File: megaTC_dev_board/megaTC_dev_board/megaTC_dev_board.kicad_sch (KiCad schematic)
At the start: 20 parts, among them J1 Screw_Terminal_01x02, J10 Screw_Terminal_01x02, J11 Conn_01x06_Pin, J12 Screw_Terminal_01x02, J2 Screw_Terminal_01x02, J3 Screw_Terminal_01x02, J4 Screw_Terminal_01x02, J5 Screw_Terminal_01x02, J6 Screw_Terminal_01x02, J7 Screw_Terminal_01x02, J8 Screw_Terminal_01x02, J9 Screw_Terminal_01x02, U1 LTC2984CLX-PBF

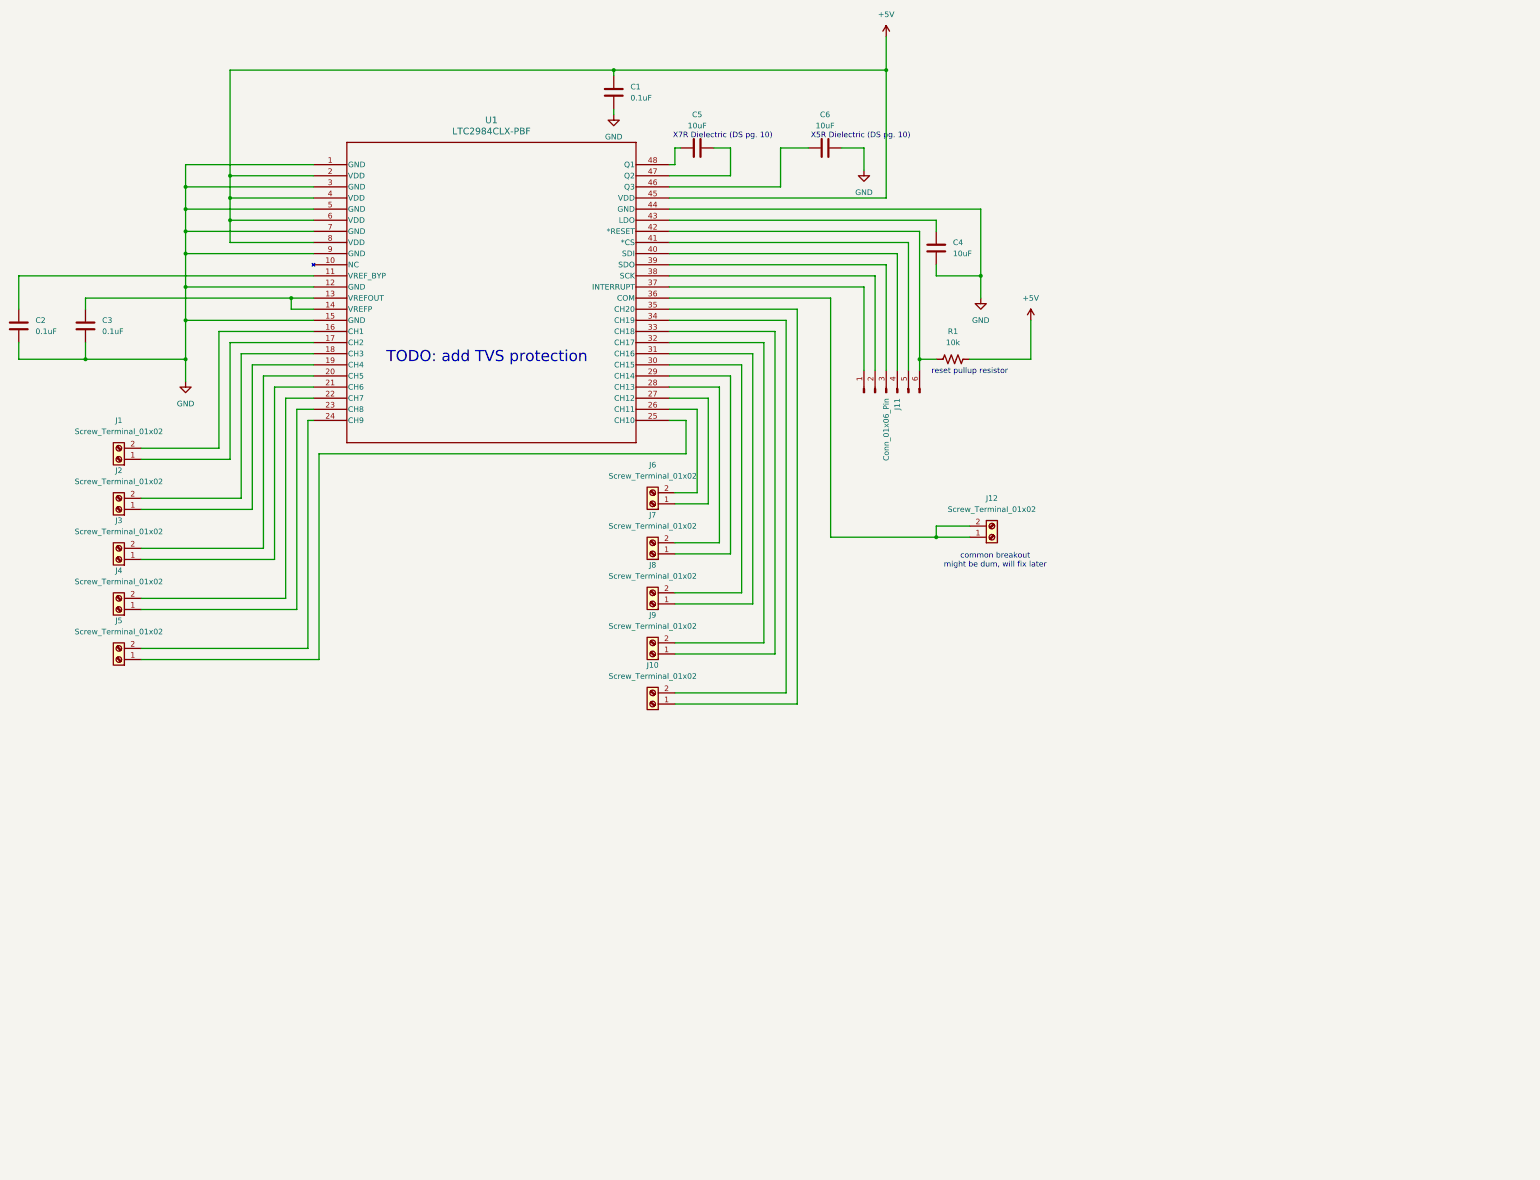
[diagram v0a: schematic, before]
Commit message: added TVS diodes, ready for routing
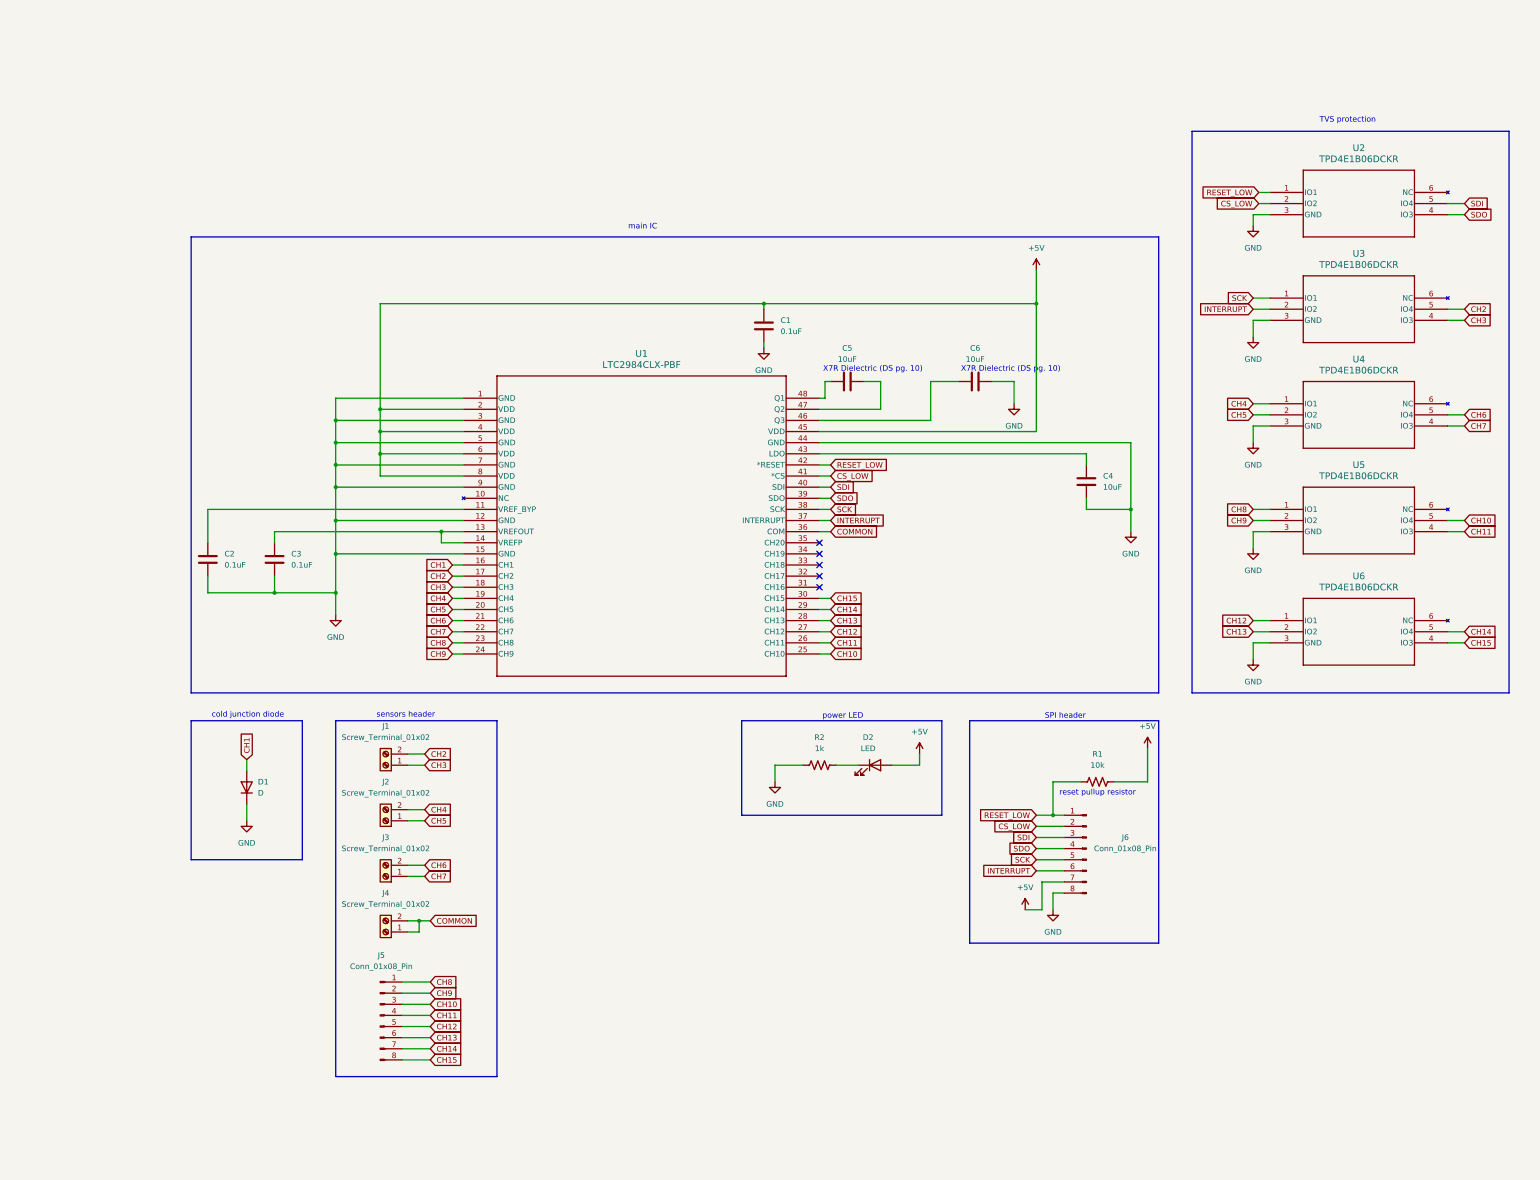
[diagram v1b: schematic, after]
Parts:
- removed J10, J12, J5, J6, J7, J8, J9: Screw_Terminal_01x02, symbol Connector:Screw_Terminal_01x02
- removed J11: Conn_01x06_Pin, symbol Connector:Conn_01x06_Pin
- added D1: D, Diode_SMD:D_0603_1608Metric, symbol Device:D
- added D2: LED, LED_SMD:LED_0603_1608Metric, symbol Device:LED
- added J5, J6: Conn_01x08_Pin, Connector_PinHeader_2.54mm:PinHeader_1x08_P2.54mm_Horizontal, symbol Connector:Conn_01x08_Pin
- added R2: 1k, Resistor_SMD:R_0603_1608Metric, symbol Device:R_US
- added U2, U3, U4, U5, U6: TPD4E1B06DCKR, DCK6_TEX, symbol TPD4E1B06DCKR:TPD4E1B06DCKR
- C1, C2, C3, C4, C5, C6: footprint (none) -> Capacitor_SMD:C_0603_1608Metric
- R1: footprint (none) -> Resistor_SMD:R_0603_1608Metric
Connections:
- net +5V: now also R1.1, D2.2 (A), J6.7 (Pin_7); no longer R1.2
- net GND: now also D1.1 (K), J6.8 (Pin_8), R2.1, U2.3 (GND), U3.3 (GND), U4.3 (GND), U5.3 (GND), U6.3 (GND)
- net RESET_LOW: now reaches U1.42 (*RESET)
- net RESET_LOW: now also R1.2, J6.1 (Pin_1), U2.1 (IO1); no longer R1.1
- net COMMON: now reaches U1.36 (COM)
- net COMMON: now also J4.1 (Pin_1), J4.2 (Pin_2)
- net CH1: now reaches U1.16 (CH1)
- net CH1: now also D1.2 (A); no longer J1.2 (Pin_2)
- net CH2: now reaches U1.17 (CH2)
- net CH2: now also J1.2 (Pin_2), U3.5 (IO4); no longer J1.1 (Pin_1)
- net CH3: now reaches U1.18 (CH3)
- net CH3: now also J1.1 (Pin_1), U3.4 (IO3); no longer J2.2 (Pin_2)
- net CH4: now reaches U1.19 (CH4)
- net CH4: now also J2.2 (Pin_2), U4.1 (IO1); no longer J2.1 (Pin_1)
- net CH5: now reaches U1.20 (CH5)
- net CH5: now also J2.1 (Pin_1), U4.2 (IO2); no longer J3.2 (Pin_2)
- net CH6: now reaches U1.21 (CH6)
- net CH6: now also J3.2 (Pin_2), U4.5 (IO4); no longer J3.1 (Pin_1)
- net CH7: now reaches U1.22 (CH7)
- net CH7: now also J3.1 (Pin_1), U4.4 (IO3); no longer J4.2 (Pin_2)
- net CH8: now reaches U1.23 (CH8)
- net CH8: now also J5.1 (Pin_1), U5.1 (IO1); no longer J4.1 (Pin_1)
- net CH9: now reaches U1.24 (CH9)
- net CH9: now also J5.2 (Pin_2), U5.2 (IO2)
- net CH10: now reaches U1.25 (CH10)
- net CH10: now also J5.3 (Pin_3), U5.5 (IO4)
- net CH11: now reaches U1.26 (CH11)
- net CH11: now also J5.4 (Pin_4), U5.4 (IO3)
- net CH12: now reaches U1.27 (CH12)
- net CH12: now also J5.5 (Pin_5), U6.1 (IO1)
- net CH13: now reaches U1.28 (CH13)
- net CH13: now also J5.6 (Pin_6), U6.2 (IO2)
- net CH14: now reaches U1.29 (CH14)
- net CH14: now also J5.7 (Pin_7), U6.5 (IO4)
- net CH15: now reaches U1.30 (CH15)
- net CH15: now also J5.8 (Pin_8), U6.4 (IO3)
- net INTERRUPT: now reaches U1.37 (INTERRUPT)
- net INTERRUPT: now also J6.6 (Pin_6), U3.2 (IO2)
- net SCK: now reaches U1.38 (SCK)
- net SCK: now also J6.5 (Pin_5), U3.1 (IO1)
- net SDO: now reaches U1.39 (SDO)
- net SDO: now also J6.4 (Pin_4), U2.4 (IO3)
- net SDI: now reaches U1.40 (SDI)
- net SDI: now also J6.3 (Pin_3), U2.5 (IO4)
- net CS_LOW: now reaches U1.41 (*CS)
- net CS_LOW: now also J6.2 (Pin_2), U2.2 (IO2)
- new net: D2.1 (K), R2.2
- no-connect marks 0 -> 5
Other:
- note added: "SPI header"
- note added: "TVS protection"
- note added: "cold junction diode"
- note added: "main IC"
- note added: "power LED"
- note added: "sensors header"
- note removed: "TODO: add TVS protection"
- note removed: "X5R Dielectric (DS pg. 10)"
- note removed: "common breakout might be dum, will fix later"
- moved on the sheet: C1, C2, C3, C4, C5, C6, J1, J2, J3, R1, U1

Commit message: started layout
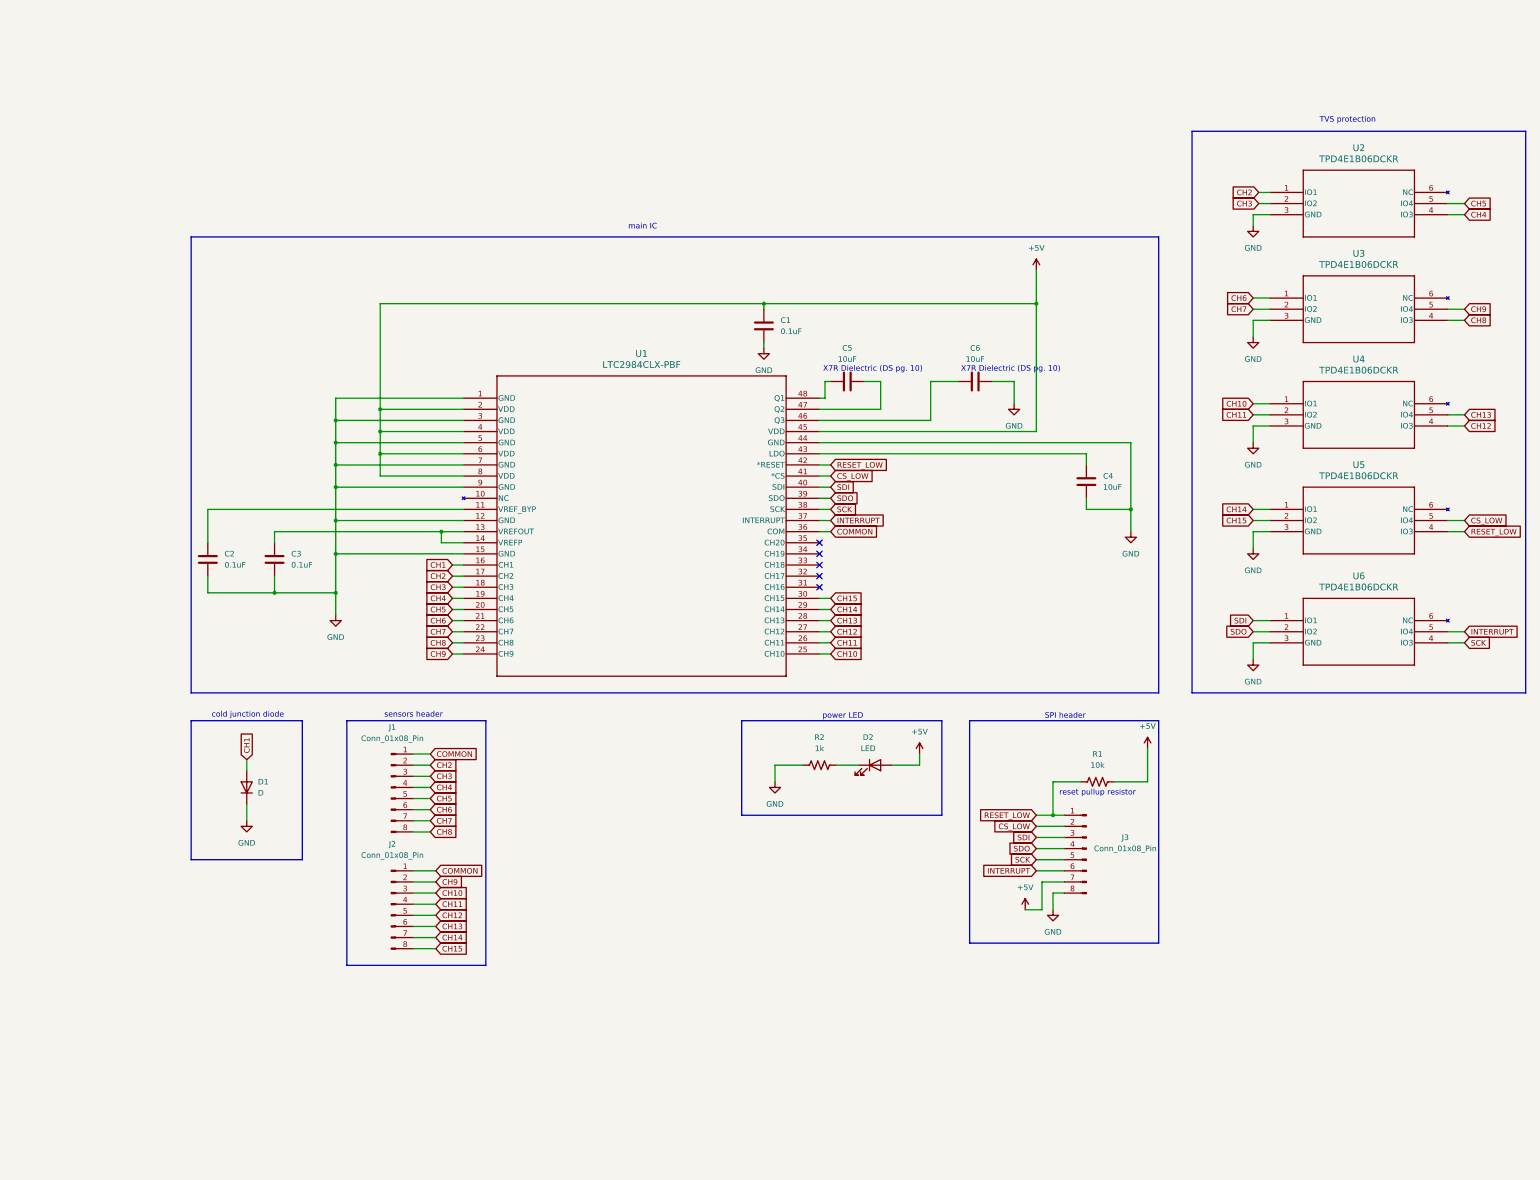
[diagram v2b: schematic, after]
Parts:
- removed J1, J2, J3, J4: Screw_Terminal_01x02, symbol Connector:Screw_Terminal_01x02
- added J1: Conn_01x08_Pin, Connector_PinHeader_2.54mm:PinHeader_1x08_P2.54mm_Vertical, symbol Connector:Conn_01x08_Pin
- J2: renamed from J5; footprint Connector_PinHeader_2.54mm:PinHeader_1x08_P2.54mm_Horizontal -> Connector_PinHeader_2.54mm:PinHeader_1x08_P2.54mm_Vertical
- J3: renamed from J6; footprint Connector_PinHeader_2.54mm:PinHeader_1x08_P2.54mm_Horizontal -> Connector_PinHeader_2.54mm:PinHeader_1x08_P2.54mm_Vertical
- U1: footprint LQFP-48_LX_LIT -> avi_footprint:LQFP-48_LX_LIT
- U2, U3, U4, U5, U6: footprint DCK6_TEX -> avi_footprint:DCK6_TEX
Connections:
- net CH10: now also U4.1 (IO1); no longer U5.5 (IO4)
- net CH11: now also U4.2 (IO2); no longer U5.4 (IO3)
- net CH12: now also U4.4 (IO3); no longer U6.1 (IO1)
- net CH13: now also U4.5 (IO4); no longer U6.2 (IO2)
- net CH14: now also U5.1 (IO1); no longer U6.5 (IO4)
- net CH15: now also U5.2 (IO2); no longer U6.4 (IO3)
- net CH2: now also U2.1 (IO1), J1.2 (Pin_2); no longer U3.5 (IO4)
- net CH3: now also U2.2 (IO2), J1.3 (Pin_3); no longer U3.4 (IO3)
- net CH4: now also U2.4 (IO3), J1.4 (Pin_4); no longer U4.1 (IO1)
- net CH5: now also U2.5 (IO4), J1.5 (Pin_5); no longer U4.2 (IO2)
- net CH6: now also U3.1 (IO1), J1.6 (Pin_6); no longer U4.5 (IO4)
- net CH7: now also U3.2 (IO2), J1.7 (Pin_7); no longer U4.4 (IO3)
- net CH8: now also U3.4 (IO3), J1.8 (Pin_8); no longer J2.1 (Pin_1), U5.1 (IO1)
- net CH9: now also U3.5 (IO4); no longer U5.2 (IO2)
- net COMMON: now also J2.1 (Pin_1), J1.1 (Pin_1)
- net CS_LOW: now also U5.5 (IO4); no longer U2.2 (IO2)
- net INTERRUPT: now also U6.5 (IO4); no longer U3.2 (IO2)
- net RESET_LOW: now also U5.4 (IO3); no longer U2.1 (IO1)
- net SCK: now also U6.4 (IO3); no longer U3.1 (IO1)
- net SDI: now also U6.1 (IO1); no longer U2.5 (IO4)
- net SDO: now also U6.2 (IO2); no longer U2.4 (IO3)
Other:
- moved on the sheet: J2

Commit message: routing routingghsdjadsd
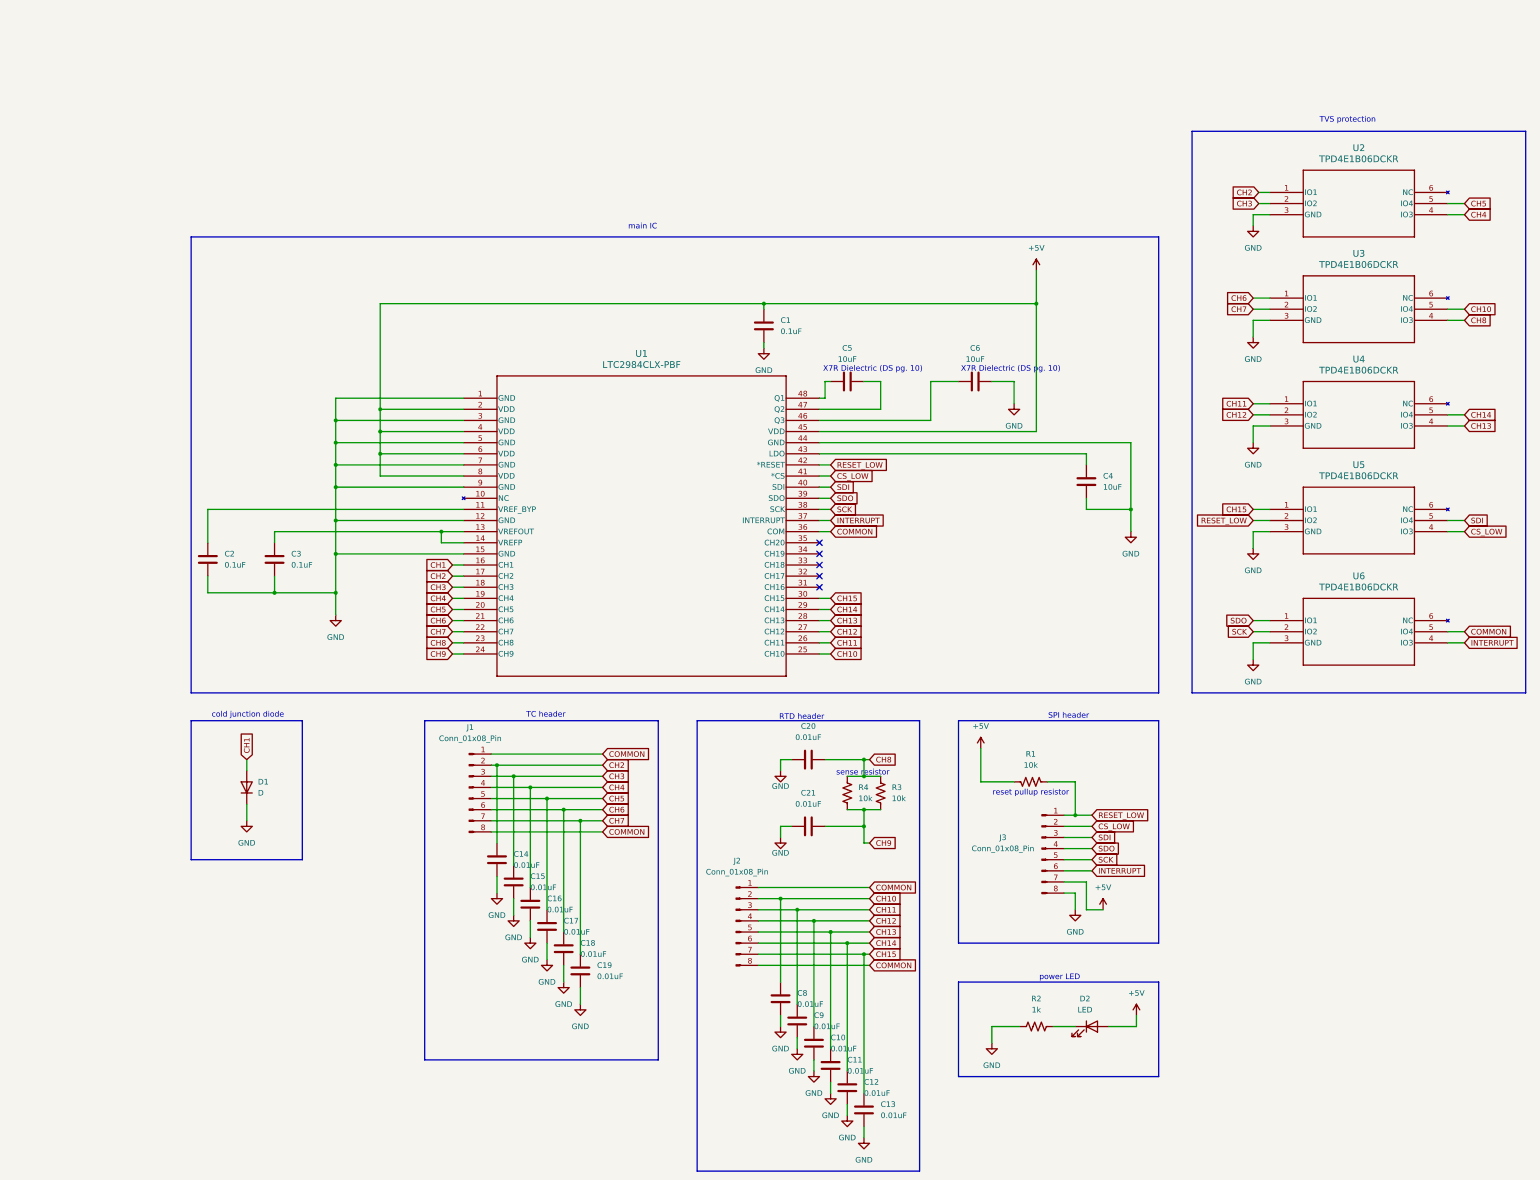
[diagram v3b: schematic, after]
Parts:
- added C10, C11, C12, C13, C14, C15, C16, C17, C18, C19, C20, C21, C8, C9: 0.01uF, Capacitor_SMD:C_0603_1608Metric, symbol Device:C
- added R3, R4: 10k, Resistor_SMD:R_0603_1608Metric, symbol Device:R_US
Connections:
- net CH10: now also J2.2 (Pin_2), U3.5 (IO4), C8.1; no longer J2.3 (Pin_3), U4.1 (IO1)
- net CH11: now also J2.3 (Pin_3), U4.1 (IO1), C9.1; no longer J2.4 (Pin_4), U4.2 (IO2)
- net CH12: now also J2.4 (Pin_4), U4.2 (IO2), C10.1; no longer J2.5 (Pin_5), U4.4 (IO3)
- net CH13: now also J2.5 (Pin_5), U4.4 (IO3), C11.1; no longer J2.6 (Pin_6), U4.5 (IO4)
- net CH14: now also J2.6 (Pin_6), U4.5 (IO4), C12.1; no longer J2.7 (Pin_7), U5.1 (IO1)
- net CH15: now also J2.7 (Pin_7), U5.1 (IO1), C13.1; no longer J2.8 (Pin_8), U5.2 (IO2)
- net CH2: now also C14.1
- net CH3: now also C15.1
- net CH4: now also C16.1
- net CH5: now also C17.1
- net CH6: now also C18.1
- net CH7: now also C19.1
- net CH8: now also C20.1, R3.1, R4.1; no longer J1.8 (Pin_8)
- net CH9: now also C21.1, R3.2, R4.2; no longer J2.2 (Pin_2), U3.5 (IO4)
- net COMMON: now also J1.8 (Pin_8), J2.8 (Pin_8), U6.5 (IO4)
- net CS_LOW: now also U5.4 (IO3); no longer U5.5 (IO4)
- net GND: now also C10.2, C11.2, C12.2, C13.2, C14.2, C15.2, C16.2, C17.2, C18.2, C19.2, C20.2, C21.2, C8.2, C9.2
- net INTERRUPT: now also U6.4 (IO3); no longer U6.5 (IO4)
- net RESET_LOW: now also U5.2 (IO2); no longer U5.4 (IO3)
- net SCK: now also U6.2 (IO2); no longer U6.4 (IO3)
- net SDI: now also U5.5 (IO4); no longer U6.1 (IO1)
- net SDO: now also U6.1 (IO1); no longer U6.2 (IO2)
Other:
- note added: "RTD header"
- note added: "TC header"
- note added: "sense resistor"
- note removed: "sensors header"
- moved on the sheet: D2, J1, J2, J3, R1, R2
